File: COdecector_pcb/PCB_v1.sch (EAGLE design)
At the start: 44 parts, among them IC2 FT230XS, IC3 AD708, X1 MINI-USB-32005-301

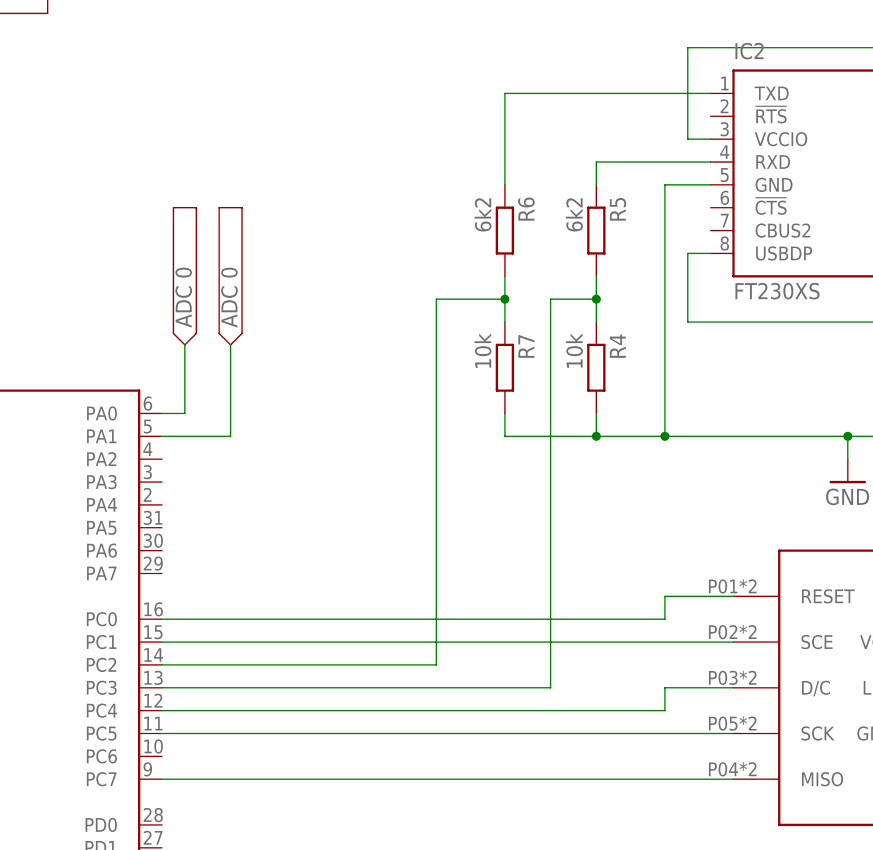
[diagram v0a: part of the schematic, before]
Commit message: Start with layout
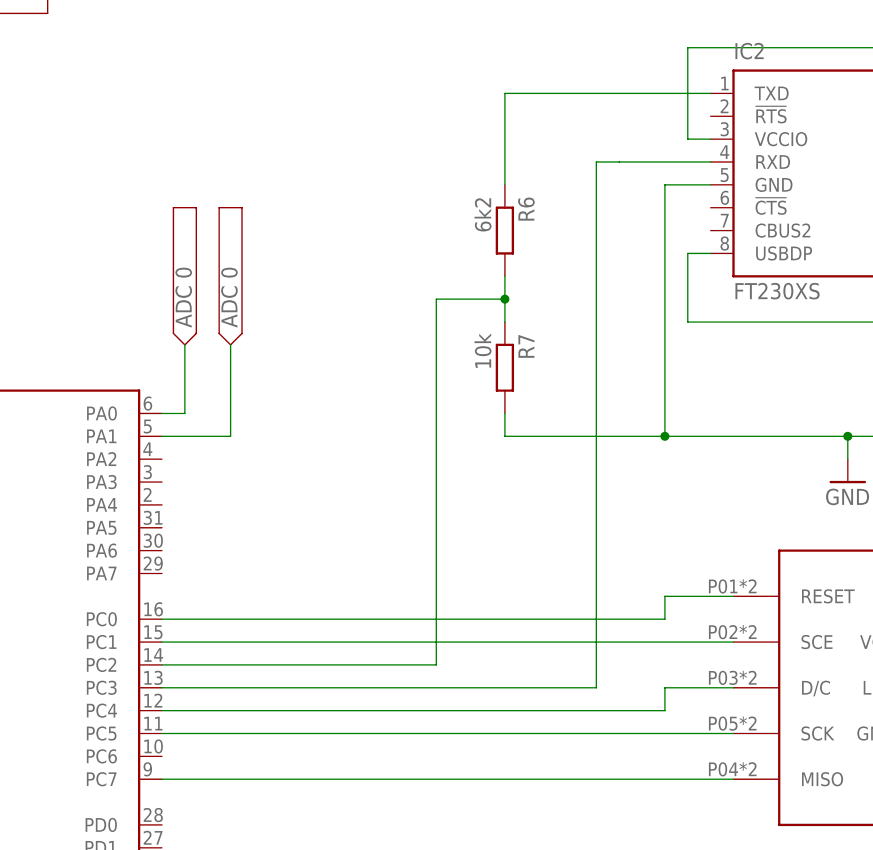
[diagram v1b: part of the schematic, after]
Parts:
- removed R4: 10k, eagle-ltspice:RR3216
- removed R5: 6k2, eagle-ltspice:RR3216
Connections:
- removed net N$18: IC2.RXD, R5.1
- net GND: no longer R4.2
- net N$19: now also IC2.RXD; no longer R4.1, R5.2
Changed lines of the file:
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@@
 <part name="L2" library="rcl" deviceset="L-US" device="L2012C" value="1m"/>
 <part name="SUPPLY4" library="supply2" deviceset="VCC" device="" value="VCC USB"/>
-<part name="R4" library="eagle-ltspice" deviceset="R" device="R3216" value="10k"/>
-<part name="R5" library="eagle-ltspice" deviceset="R" device="R3216" value="6k2"/>
 <part name="R6" library="eagle-ltspice" deviceset="R" device="R3216" value="6k2"/>
 <part name="R7" library="eagle-ltspice" deviceset="R" device="R3216" value="10k"/>
@@
 <instance part="L2" gate="G$1" x="226.06" y="134.62" rot="R90"/>
 <instance part="SUPPLY4" gate="G$1" x="208.28" y="177.8"/>
-<instance part="R4" gate="G$1" x="144.78" y="114.3" rot="R270"/>
-<instance part="R5" gate="G$1" x="144.78" y="129.54" rot="R270"/>
 <instance part="R6" gate="G$1" x="134.62" y="129.54" rot="R270"/>
 <instance part="R7" gate="G$1" x="134.62" y="114.3" rot="R270"/>
@@
 <pinref part="R7" gate="G$1" pin="2"/>
 <wire x1="134.62" y1="109.22" x2="134.62" y2="106.68" width="0.1524" layer="91"/>
-<pinref part="R4" gate="G$1" pin="2"/>
-<wire x1="134.62" y1="106.68" x2="144.78" y2="106.68" width="0.1524" layer="91"/>
-<wire x1="144.78" y1="106.68" x2="144.78" y2="109.22" width="0.1524" layer="91"/>
-<wire x1="144.78" y1="106.68" x2="152.4" y2="106.68" width="0.1524" layer="91"/>
-<junction x="144.78" y="106.68"/>
+<wire x1="134.62" y1="106.68" x2="152.4" y2="106.68" width="0.1524" layer="91"/>
 <junction x="152.4" y="106.68"/>
 <pinref part="C7" gate="G$1" pin="2"/>
@@
 </segment>
 </net>
-<net name="N$18" class="0">
-<segment>
-<pinref part="IC2" gate="G$1" pin="RXD"/>
-<wire x1="157.48" y1="137.16" x2="144.78" y2="137.16" width="0.1524" layer="91"/>
-<pinref part="R5" gate="G$1" pin="1"/>
-<wire x1="144.78" y1="134.62" x2="144.78" y2="137.16" width="0.1524" layer="91"/>
-</segment>
-</net>
 <net name="N$17" class="0">
 <segment>
@@
 <net name="N$19" class="0">
 <segment>
-<pinref part="R4" gate="G$1" pin="1"/>
-<pinref part="R5" gate="G$1" pin="2"/>
-<wire x1="144.78" y1="119.38" x2="144.78" y2="121.92" width="0.1524" layer="91"/>
 <pinref part="IC1" gate="G$1" pin="PC3"/>
-<wire x1="144.78" y1="121.92" x2="144.78" y2="124.46" width="0.1524" layer="91"/>
-<wire x1="139.7" y1="78.74" x2="96.52" y2="78.74" width="0.1524" layer="91"/>
-<wire x1="144.78" y1="121.92" x2="139.7" y2="121.92" width="0.1524" layer="91"/>
-<wire x1="139.7" y1="121.92" x2="139.7" y2="78.74" width="0.1524" layer="91"/>
-<junction x="144.78" y="121.92"/>
-</segment>
-</net>
+<wire x1="144.78" y1="78.74" x2="96.52" y2="78.74" width="0.1524" layer="91"/>
+<pinref part="IC2" gate="G$1" pin="RXD"/>
+<wire x1="157.48" y1="137.16" x2="147.32" y2="137.16" width="0.1524" layer="91"/>
+<wire x1="144.78" y1="78.74" x2="144.78" y2="137.16" width="0.1524" layer="91"/>
+<wire x1="144.78" y1="137.16" x2="147.32" y2="137.16" width="0.1524" layer="91"/>
+</segment>
+</net>
